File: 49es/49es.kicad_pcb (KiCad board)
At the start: 2 copper layers, 13 parts, among them J1 Conn_02x13_Row_Letter_Last, J2 Conn_01x04

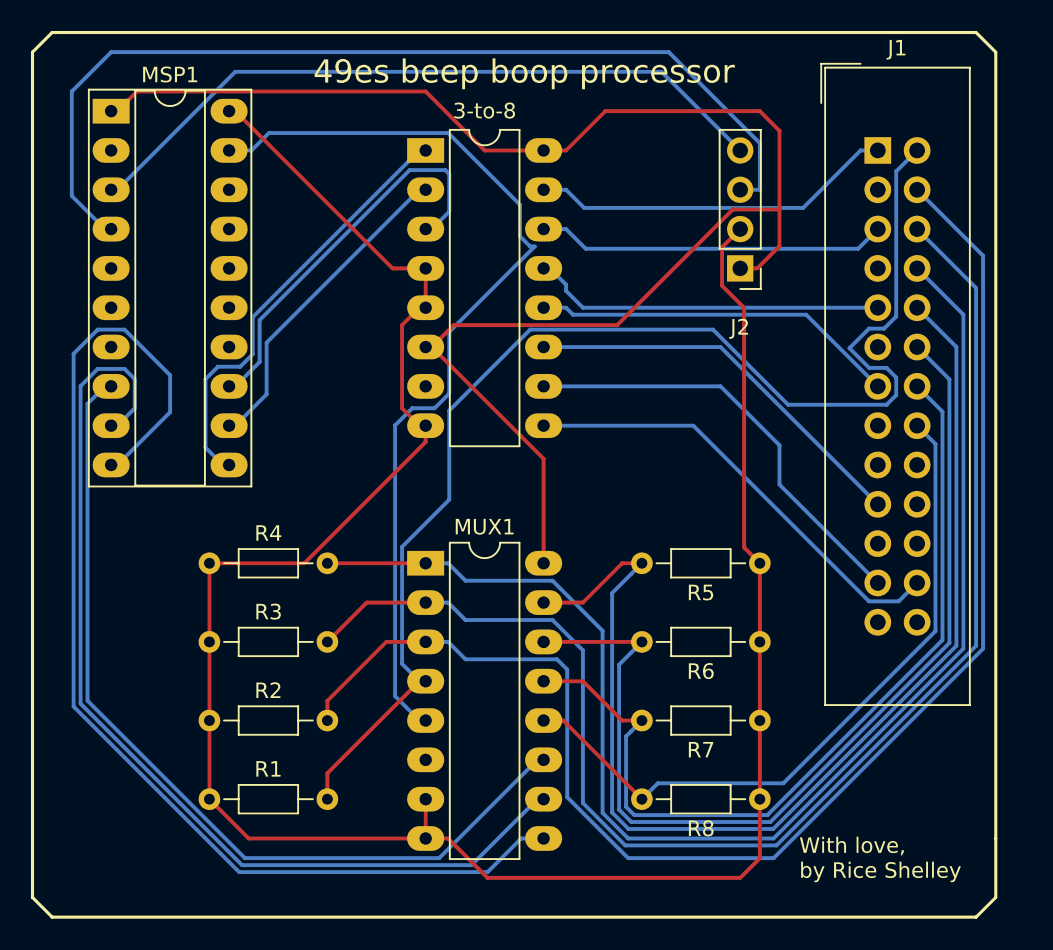
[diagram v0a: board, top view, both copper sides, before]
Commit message: welp
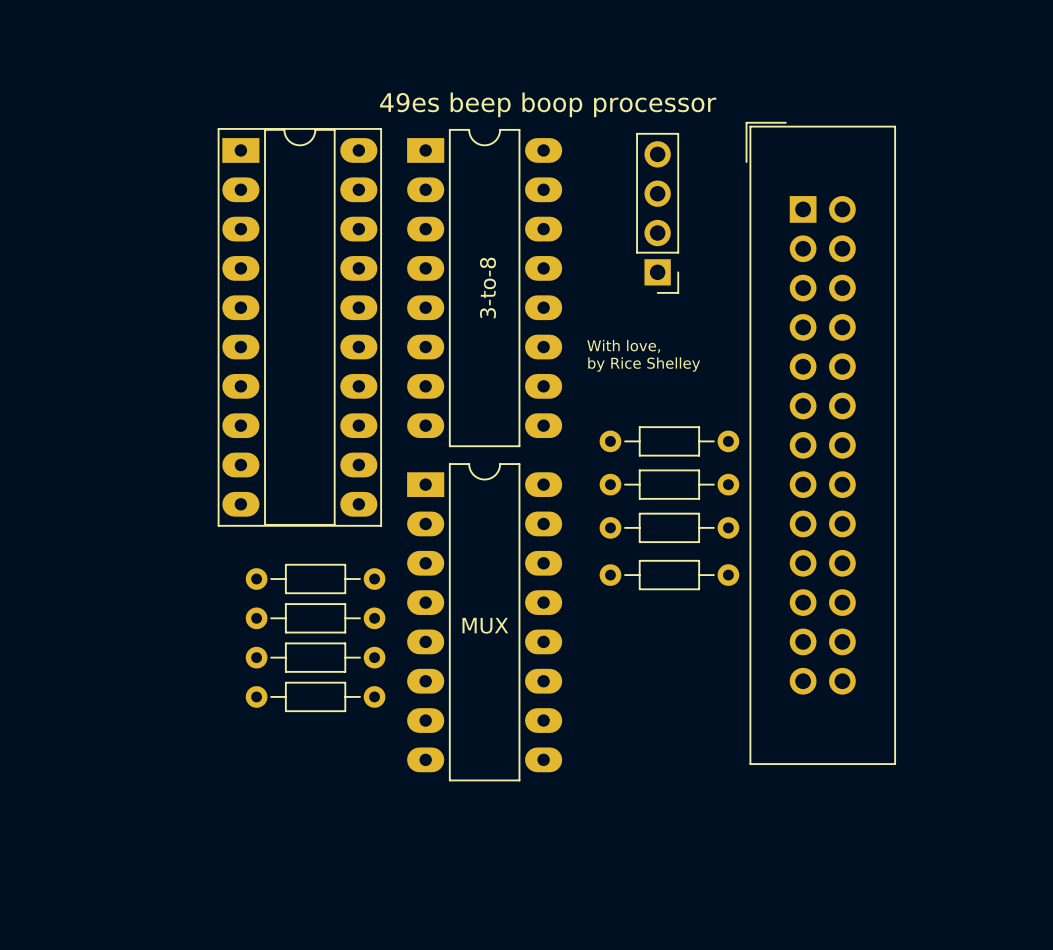
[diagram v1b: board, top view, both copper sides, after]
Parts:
- moved R8 14.6 mm to (189.7, 89.7)
- moved R7 12.6 mm to (189.7, 86.6)
- moved R6 10.4 mm to (189.7, 83.8)
- moved MSP1 8.76 mm to (158.2, 62.2)
- moved R5 8.13 mm to (189.7, 81.0)
- moved R1 7.27 mm to (159.3, 97.5)
- moved J1 6.15 mm to (194.6, 66.0)
- moved J2 5.34 mm to (185.2, 70.1)
- moved MUX 5.08 mm to (170.2, 83.8)
- moved R2 5.08 mm to (159.3, 95.0)
- moved R3 3.41 mm to (159.3, 92.5)
- moved R4 3.21 mm to (159.3, 89.9)
- renumbered MUX1 to MUX
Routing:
- net GND: track 145.2 -> 0.00 mm
- net +3V3: track 101.0 -> 0.00 mm
- net Net-(J1-Pad4): track 92.8 -> 0.00 mm
- net Net-(J1-Pad6): track 89.1 -> 0.00 mm
- net Net-(J1-Pad8): track 86.2 -> 0.00 mm
- net Net-(J1-Pad2): track 83.5 -> 0.00 mm
- net Net-(J1-Pad10): track 74.8 -> 0.00 mm
- net Net-(MSP1-Pad10): track 74.2 -> 0.00 mm
- net Net-(MSP1-Pad9): track 64.6 -> 0.00 mm
- net Net-(J1-Pad12): track 64.2 -> 0.00 mm
- net Net-(J2-Pad3): track 62.4 -> 0.00 mm
- net Net-(MSP1-Pad19): track 60.7 -> 0.00 mm
- net Net-(MSP1-Pad8): track 57.5 -> 0.00 mm
- net Net-(J1-Pad14): track 55.8 -> 0.00 mm
- net Net-(J2-Pad4): track 45.9 -> 0.00 mm
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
